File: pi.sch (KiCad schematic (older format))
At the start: 16 parts

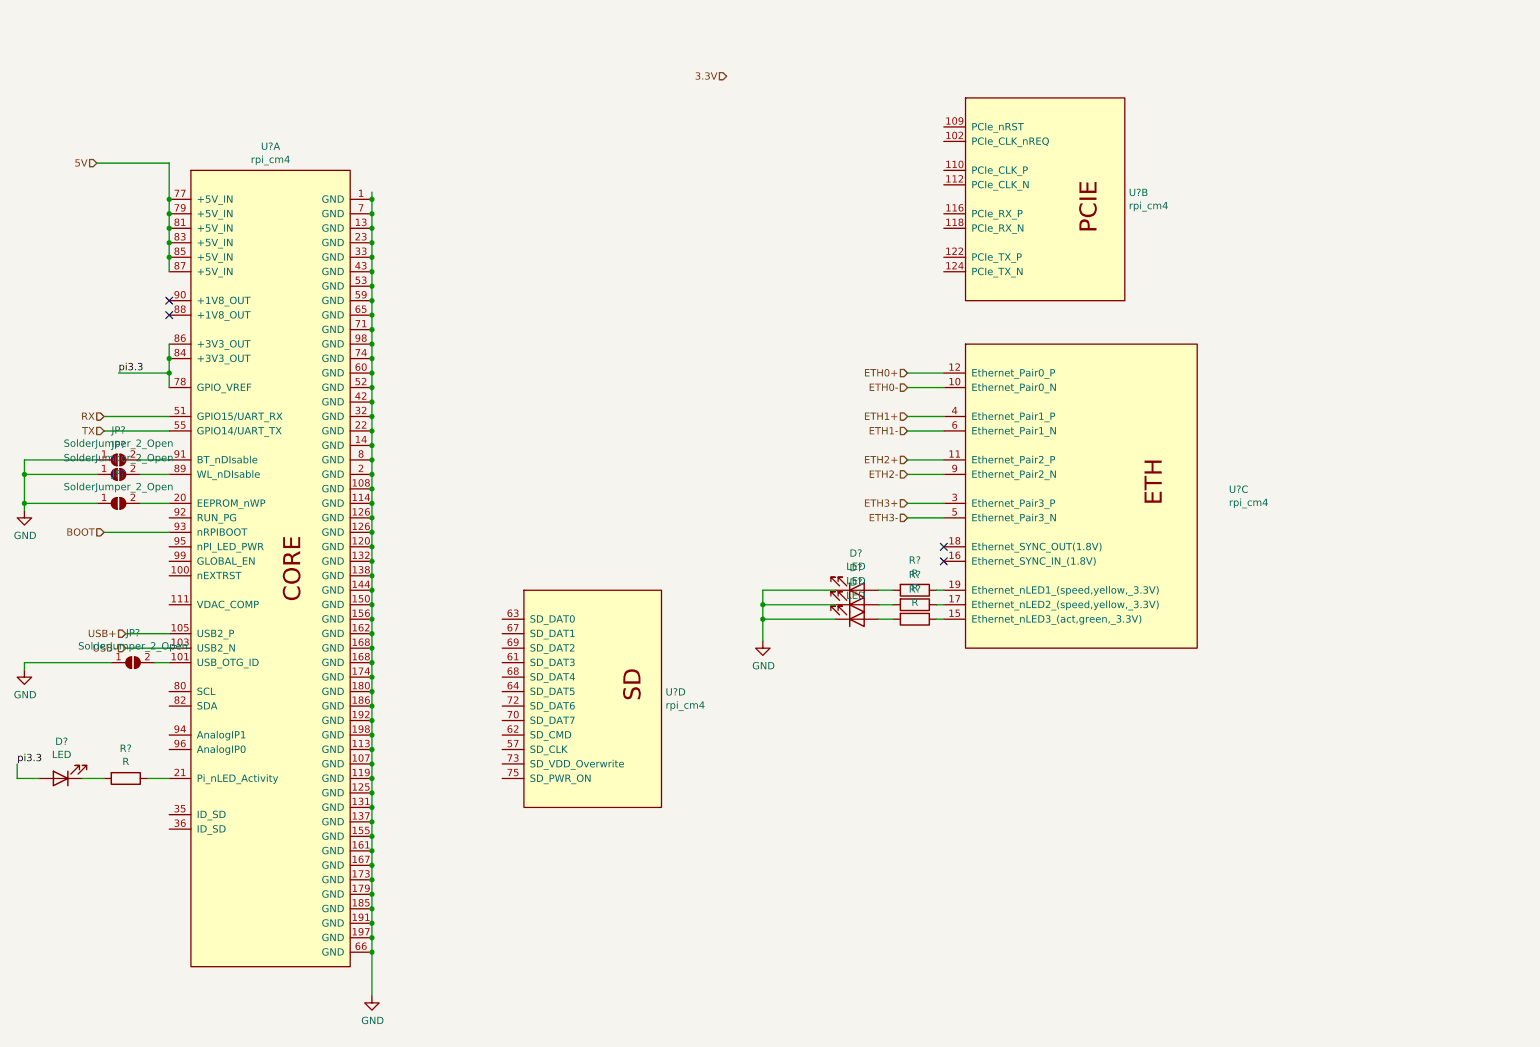
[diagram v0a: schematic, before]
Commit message: nvme
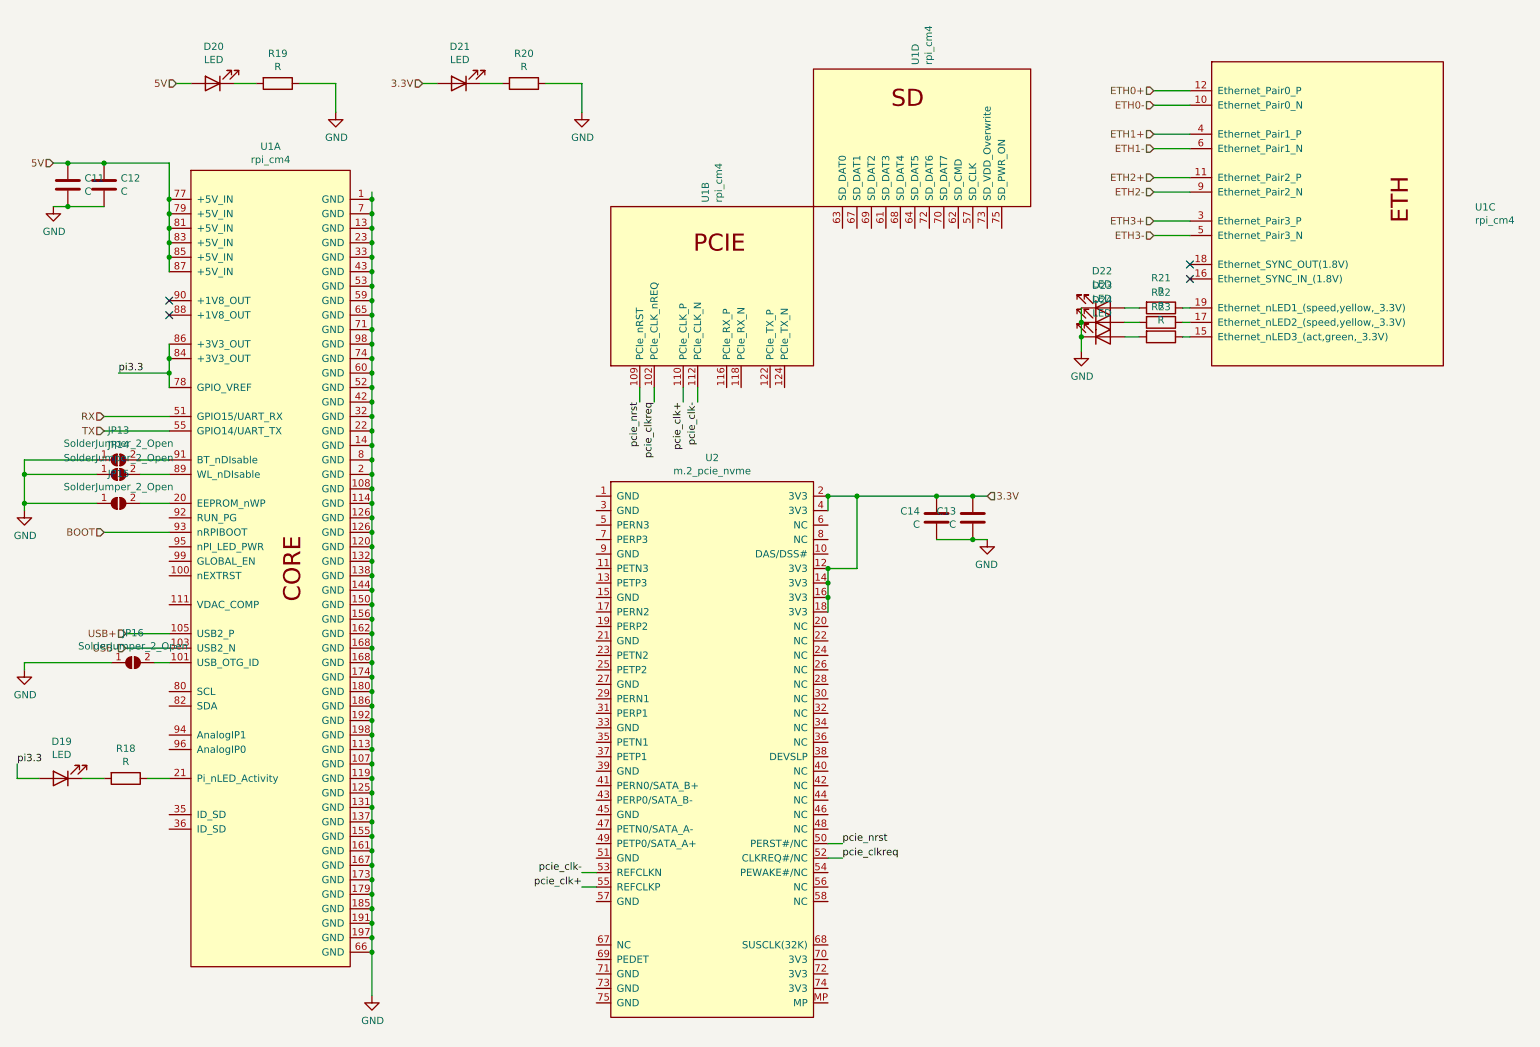
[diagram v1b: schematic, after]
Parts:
- added C1, C3: C, Capacitor_SMD:C_0805_2012Metric, symbol Device:C
- added C2, C4: C, Capacitor_SMD:C_0603_1608Metric, symbol Device:C
- added D3, D4: LED, LED_SMD:LED_0603_1608Metric, symbol Device:LED
- added R2, R3: R, Resistor_SMD:R_0603_1608Metric, symbol Device:R
- added U2: m.2_pcie_nvme, dg_connectors:m.2_pcie_nvme, symbol dg_connectors:m.2_pcie_nvme
- gave numbers to parts that had none: 13
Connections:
- net 3.3V: now also C3.1, C4.1, D4.2 (A), U2.12 (3V3), U2.14 (3V3), U2.16 (3V3), U2.18 (3V3), U2.2 (3V3), U2.4 (3V3)
- net 5V: now also C1.1, C2.1, D3.2 (A)
- net GND: now also C1.2, C2.2, C3.2, C4.2, R2.1, R3.1
- net pcie_clkreq: now reaches U1.102 (PCIe_CLK_nREQ)
- net pcie_clkreq: now also U2.52 (CLKREQ#/NC)
- net pcie_nrst: now reaches U1.109 (PCIe_nRST)
- net pcie_nrst: now also U2.50 (PERST#/NC)
- net pcie_clk+: now reaches U1.110 (PCIe_CLK_P)
- net pcie_clk+: now also U2.55 (REFCLKP)
- net pcie_clk-: now reaches U1.112 (PCIe_CLK_N)
- net pcie_clk-: now also U2.53 (REFCLKN)
- new net: D3.1 (K), R2.2
- new net: D4.1 (K), R3.2
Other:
- moved on the sheet: D22, D23, D24, R21, R22, R23, U1B, U1C, U1D

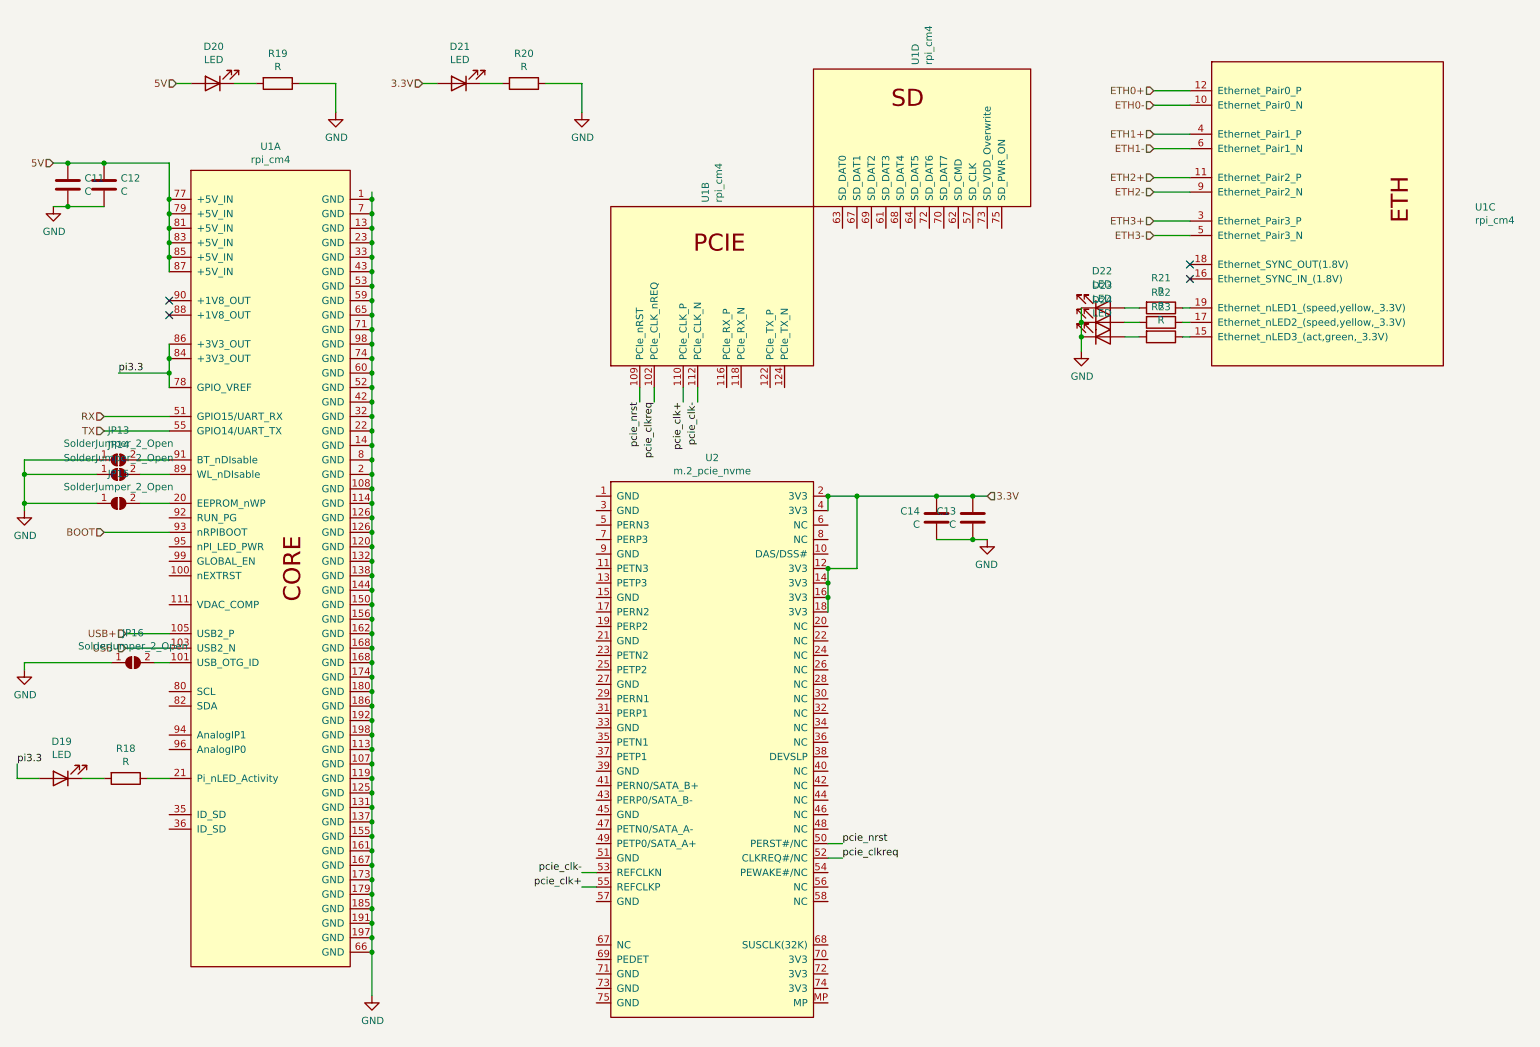
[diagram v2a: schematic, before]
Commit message: possible layout example
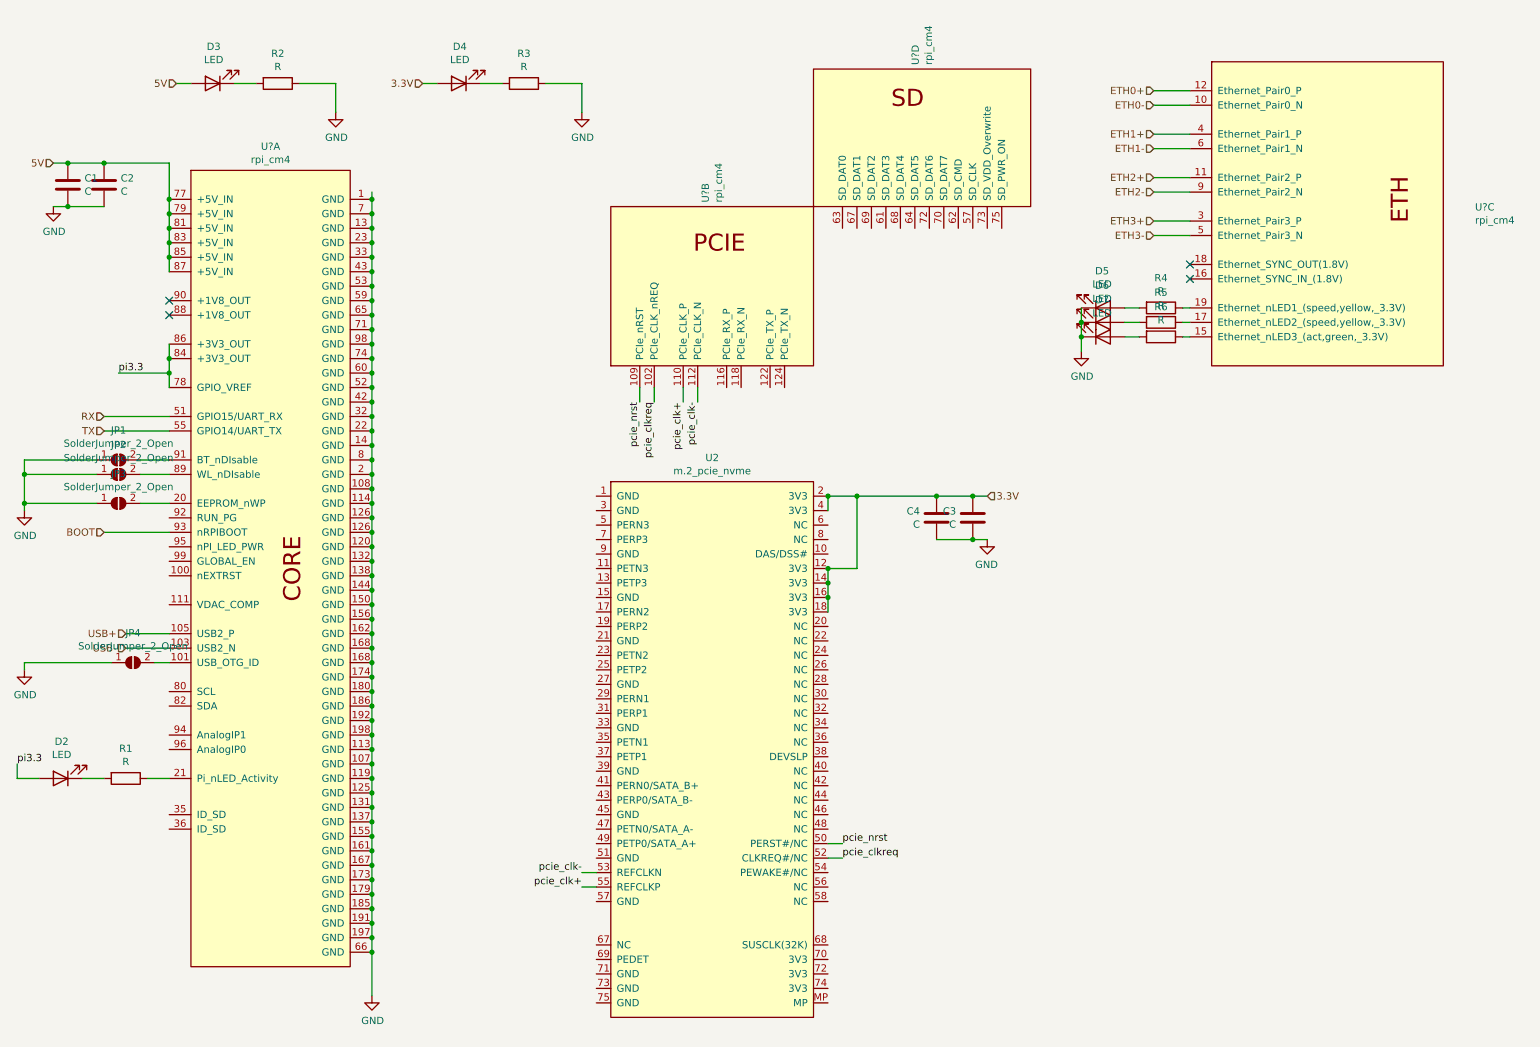
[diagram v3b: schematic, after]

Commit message: maybe use a premade powerbrick
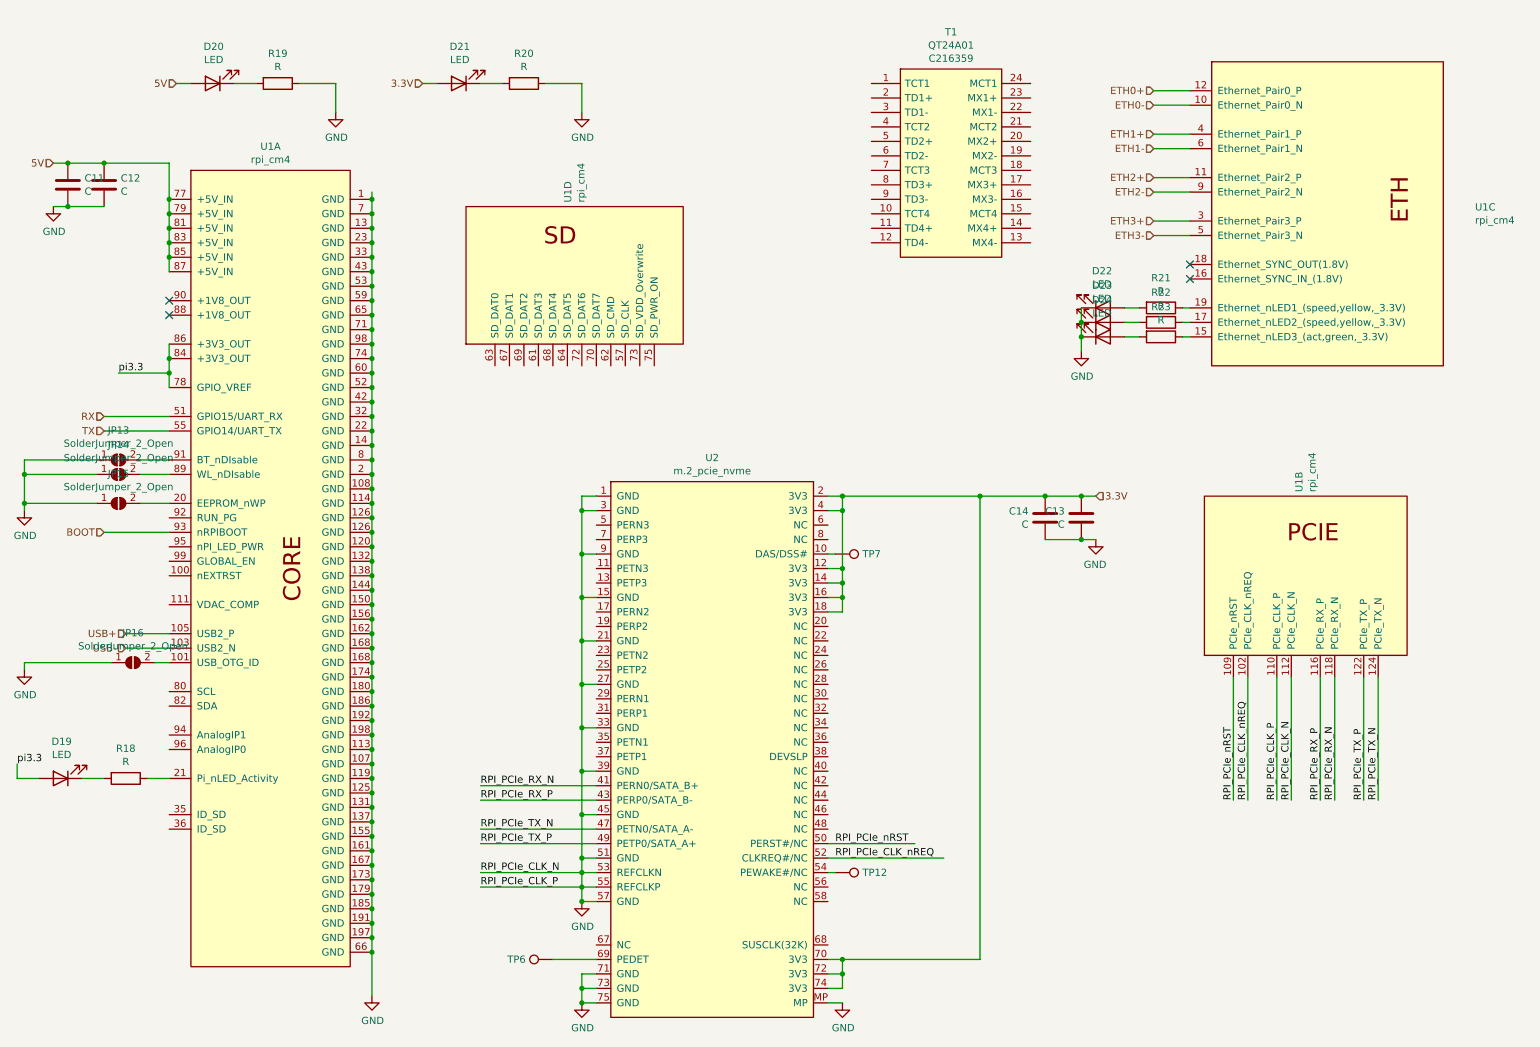
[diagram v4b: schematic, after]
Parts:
- added T2: QT24A01, dg_transformers:SOP100P1000X450-24N, symbol dg_transformers:QT24A01
- added TP13, TP14, TP15: TestPoint, TestPoint:TestPoint_Pad_D1.0mm, symbol Connector:TestPoint
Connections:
- net pcie_clk+ is gone; now on net GND: U1.110 (PCIe_CLK_P), U2.55 (REFCLKP)
- net pcie_clk- is gone; now on net GND: U1.112 (PCIe_CLK_N), U2.53 (REFCLKN)
- net 3.3V: now also U2.70 (3V3), U2.72 (3V3), U2.74 (3V3)
- net GND: now also U2.1 (GND), U2.15 (GND), U2.21 (GND), U2.27 (GND), U2.3 (GND), U2.33 (GND), U2.39 (GND), U2.45 (GND), U2.51 (GND), U2.57 (GND), U2.71 (GND), U2.73 (GND), U2.75 (GND), U2.9 (GND), U2.MP
- net RPI_PCIe_RX_P: now reaches U1.116 (PCIe_RX_P)
- net RPI_PCIe_RX_P: now also U2.43 (PERP0/SATA_B-)
- net RPI_PCIe_RX_N: now reaches U1.118 (PCIe_RX_N)
- net RPI_PCIe_RX_N: now also U2.41 (PERN0/SATA_B+)
- net RPI_PCIe_TX_P: now reaches U1.122 (PCIe_TX_P)
- net RPI_PCIe_TX_P: now also U2.49 (PETP0/SATA_A+)
- net RPI_PCIe_TX_N: now reaches U1.124 (PCIe_TX_N)
- net RPI_PCIe_TX_N: now also U2.47 (PETN0/SATA_A-)
- net at U2.10 (DAS/DSS#): now also TP14.1
- net at U2.54 (PEWAKE#/NC): now also TP15.1
- net at U2.69 (PEDET): now also TP13.1
- net pcie_clkreq renamed RPI_PCIe_CLK_nREQ
- net pcie_nrst renamed RPI_PCIe_nRST
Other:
- moved on the sheet: C13, C14, U1B, U1D
